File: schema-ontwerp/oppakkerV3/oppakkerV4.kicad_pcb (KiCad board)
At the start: 2 copper layers, 70 x 66 mm, 25 parts, among them J1 Conn_01x03, J2 Conn_01x03, J3 Conn_01x02, J6 Conn_01x04, Q1 IRLZ34N, Q2 IRLZ34N, Q3 IRLZ34N, Q4 IRLZ34N, SW1 SW_Push

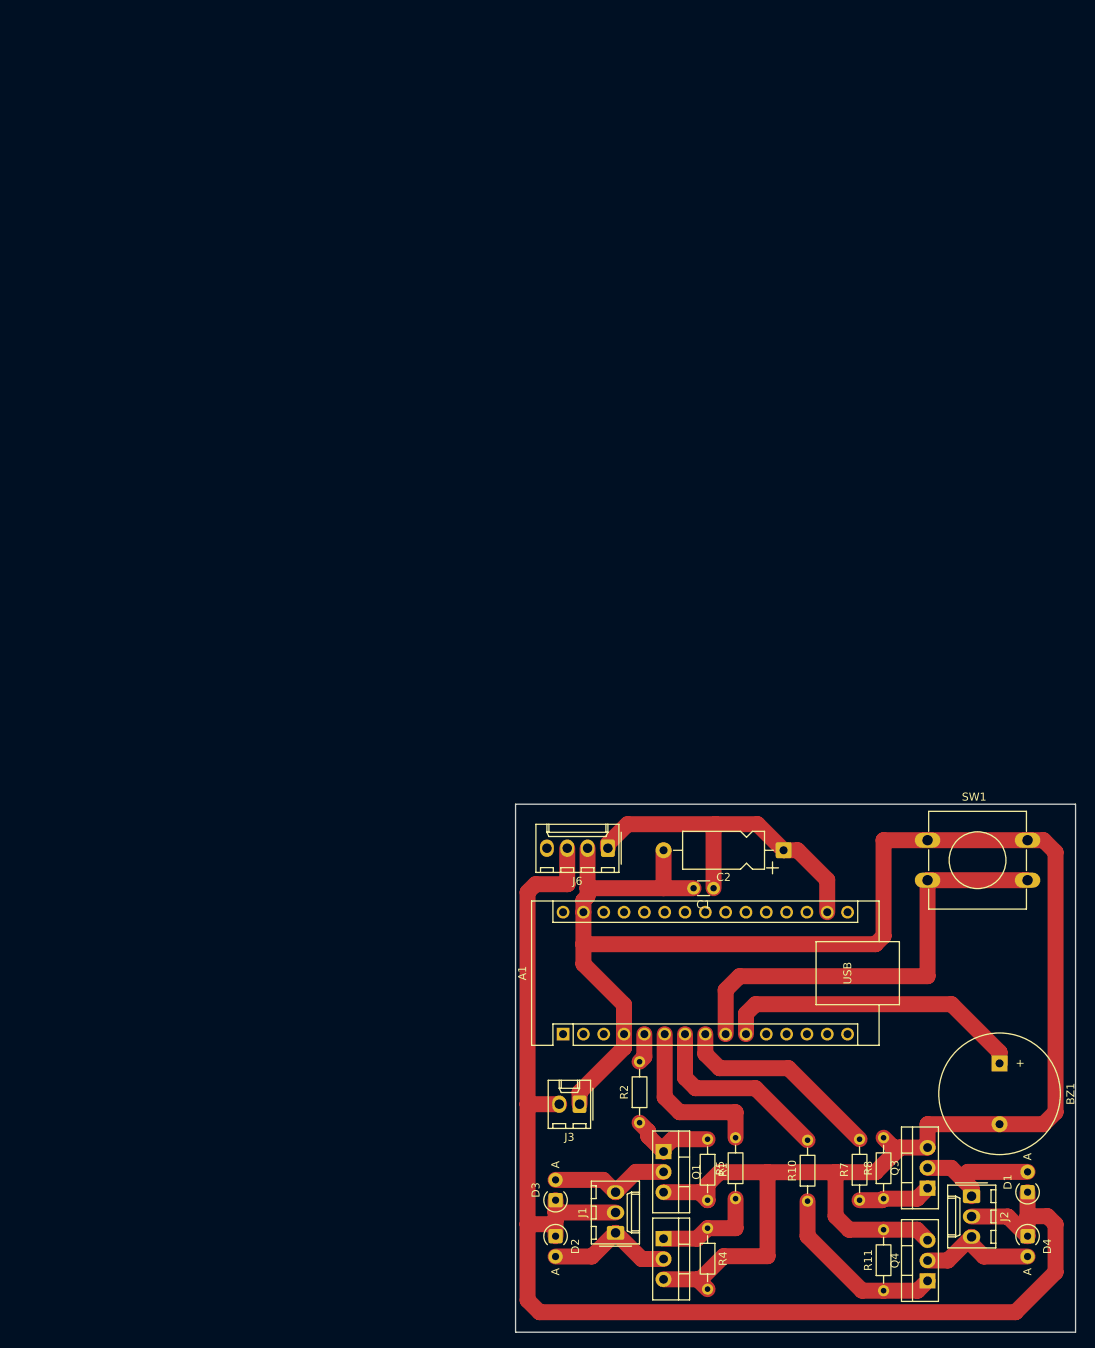
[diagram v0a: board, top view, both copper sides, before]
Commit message: update
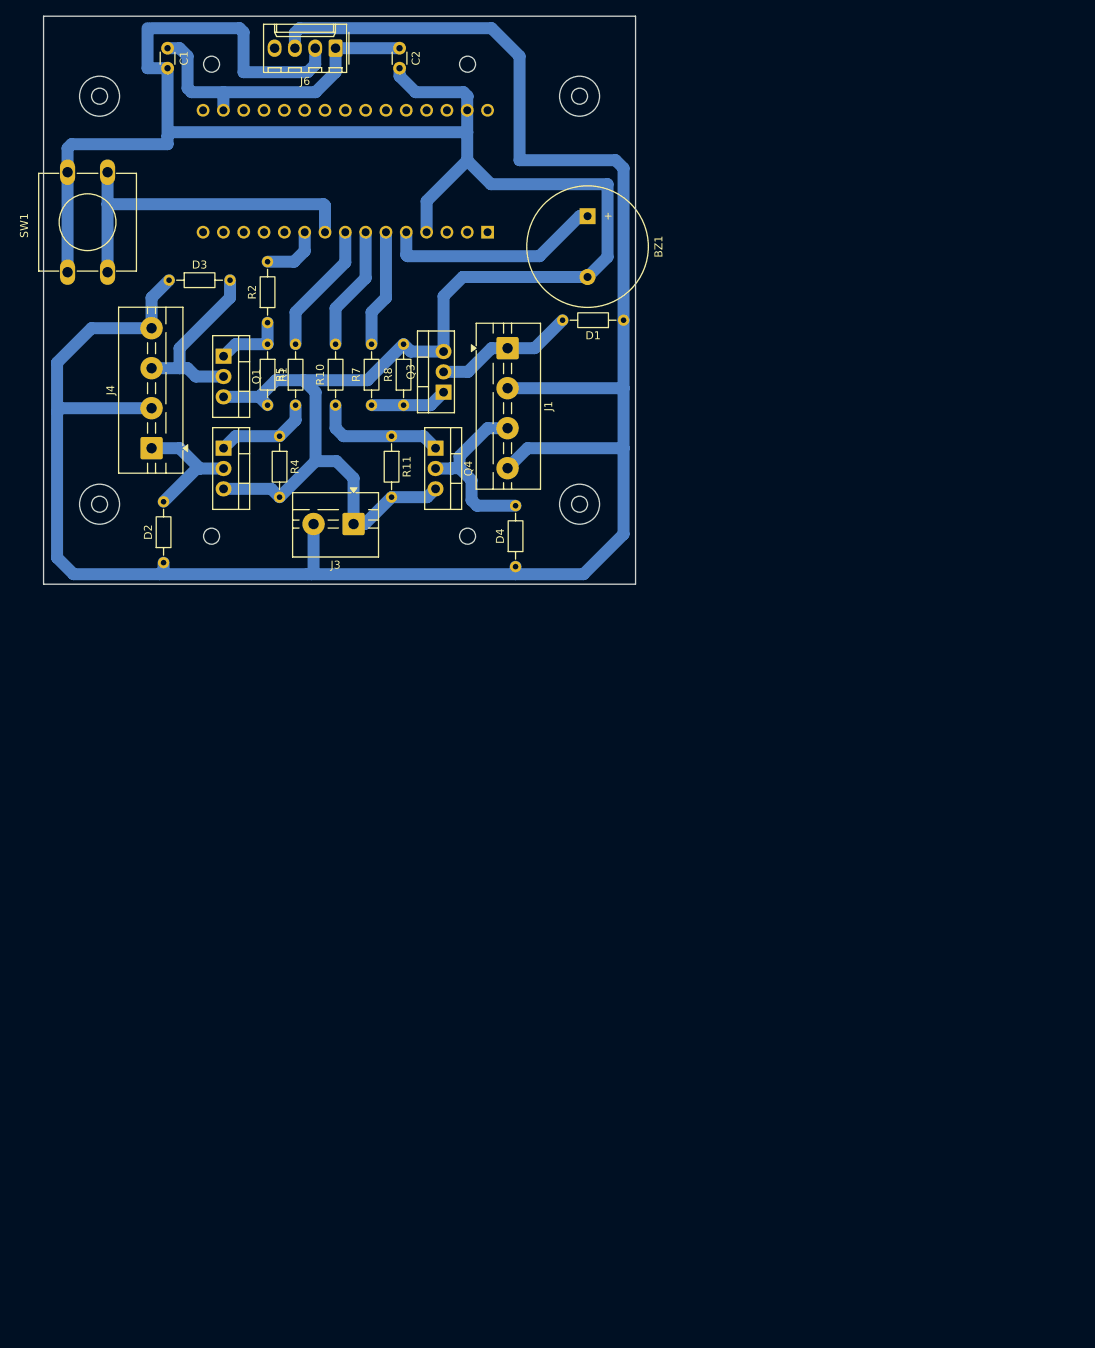
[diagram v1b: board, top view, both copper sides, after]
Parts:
- removed J2: Conn_01x03, Connector_Molex:Molex_KK-254_AE-6410-03A_1x03_P2.54mm_Vertical
- added J4: Conn_01x04, TerminalBlock:TerminalBlock_MaiXu_MX126-5.0-04P_1x04_P5.00mm, F.Cu at (38.0, 74.0)
- A1: moved to B.Cu
- C2: footprint Capacitor_THT:CP_Axial_L10.0mm_D4.5mm_P15.00mm_Horizontal -> Capacitor_THT:C_Disc_D3.0mm_W1.6mm_P2.50mm
- D1, D2, D3, D4: footprint Diode_THT:D_A-405_P2.54mm_Vertical_AnodeUp -> Resistor_THT:R_Axial_DIN0204_L3.6mm_D1.6mm_P7.62mm_Horizontal
- J1: value Conn_01x03 -> Conn_01x04; footprint Connector_Molex:Molex_KK-254_AE-6410-03A_1x03_P2.54mm_Vertical -> TerminalBlock:TerminalBlock_MaiXu_MX126-5.0-04P_1x04_P5.00mm
- J3: footprint Connector_Molex:Molex_KK-254_AE-6410-02A_1x02_P2.54mm_Vertical -> TerminalBlock:TerminalBlock_MaiXu_MX126-5.0-02P_1x02_P5.00mm
- Q1, Q2, Q3, Q4: value IRLZ34N -> IRLB8721PBF
- moved SW1 128.8 mm to (27.5, 52.0), turned to 90 degrees
- moved C1 125.2 mm to (40.0, 24.0), turned to -90 degrees
- moved D3 124.7 mm to (40.2, 53.0), turned to 0 degrees
- moved R11 123.3 mm to (68.0, 72.5), turned to -90 degrees
- moved Q4 120.9 mm to (73.5, 74.0), turned to -90 degrees
- moved D1 120.1 mm to (97.0, 58.0), turned to 180 degrees
- moved BZ1 117.8 mm to (92.5, 45.0)
- moved R7 116.6 mm to (65.5, 68.6)
- moved Q3 116.4 mm to (74.5, 67.0)
- moved R8 115.9 mm to (69.5, 68.6)
- moved R10 115.7 mm to (61.0, 68.6)
- moved Q1 113.6 mm to (47.0, 62.5)
- moved R1 113.6 mm to (52.5, 61.0)
- moved R5 113.4 mm to (56.0, 68.6)
- moved Q2 113.1 mm to (47.0, 74.0)
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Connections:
- BZ1 pad 1: Net-(A1-D7) -> Net-(A1-D2)
- J1 pad 1: Net-(D2-A) -> Net-(D1-A)
- J1 pad 3: Net-(D3-A) -> Net-(D4-A)
- R2 pad 2: Net-(A1-D2) -> Net-(A1-D7)
- R5 pad 2: Net-(A1-D3) -> Net-(A1-D5)
- R7 pad 2: Net-(A1-D5) -> Net-(A1-D3)
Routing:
- net /+48V: track 172.7 -> 273.5 mm
- net Net-(A1-D7): track 38.6 -> 7.55 mm
- net Net-(A1-D2): track 3.70 -> 27.6 mm
- net /GND: track 263.3 -> 278.0 mm
- net Net-(A1-D6): track 56.0 -> 43.1 mm
- net Net-(A1-D5): track 26.2 -> 16.6 mm
- net Net-(A1-D4): track 24.0 -> 15.6 mm
- net Net-(D3-A): track 15.2 -> 23.0 mm
- net Net-(D4-A): track 15.3 -> 22.4 mm
- net Net-(Q4-G): track 22.7 -> 16.4 mm
- net Net-(A1-D3): track 20.7 -> 14.7 mm
- net /+3.3V: track 44.0 -> 39.9 mm
- net Net-(Q1-G): track 11.2 -> 8.81 mm
- net Net-(D1-A): track 16.1 -> 17.6 mm
- net Net-(Q2-G): track 13.2 -> 12.3 mm
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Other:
- board size 70 x 66 mm -> 74 x 71 mm
